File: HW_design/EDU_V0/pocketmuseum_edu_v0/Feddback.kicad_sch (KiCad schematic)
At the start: 18 parts

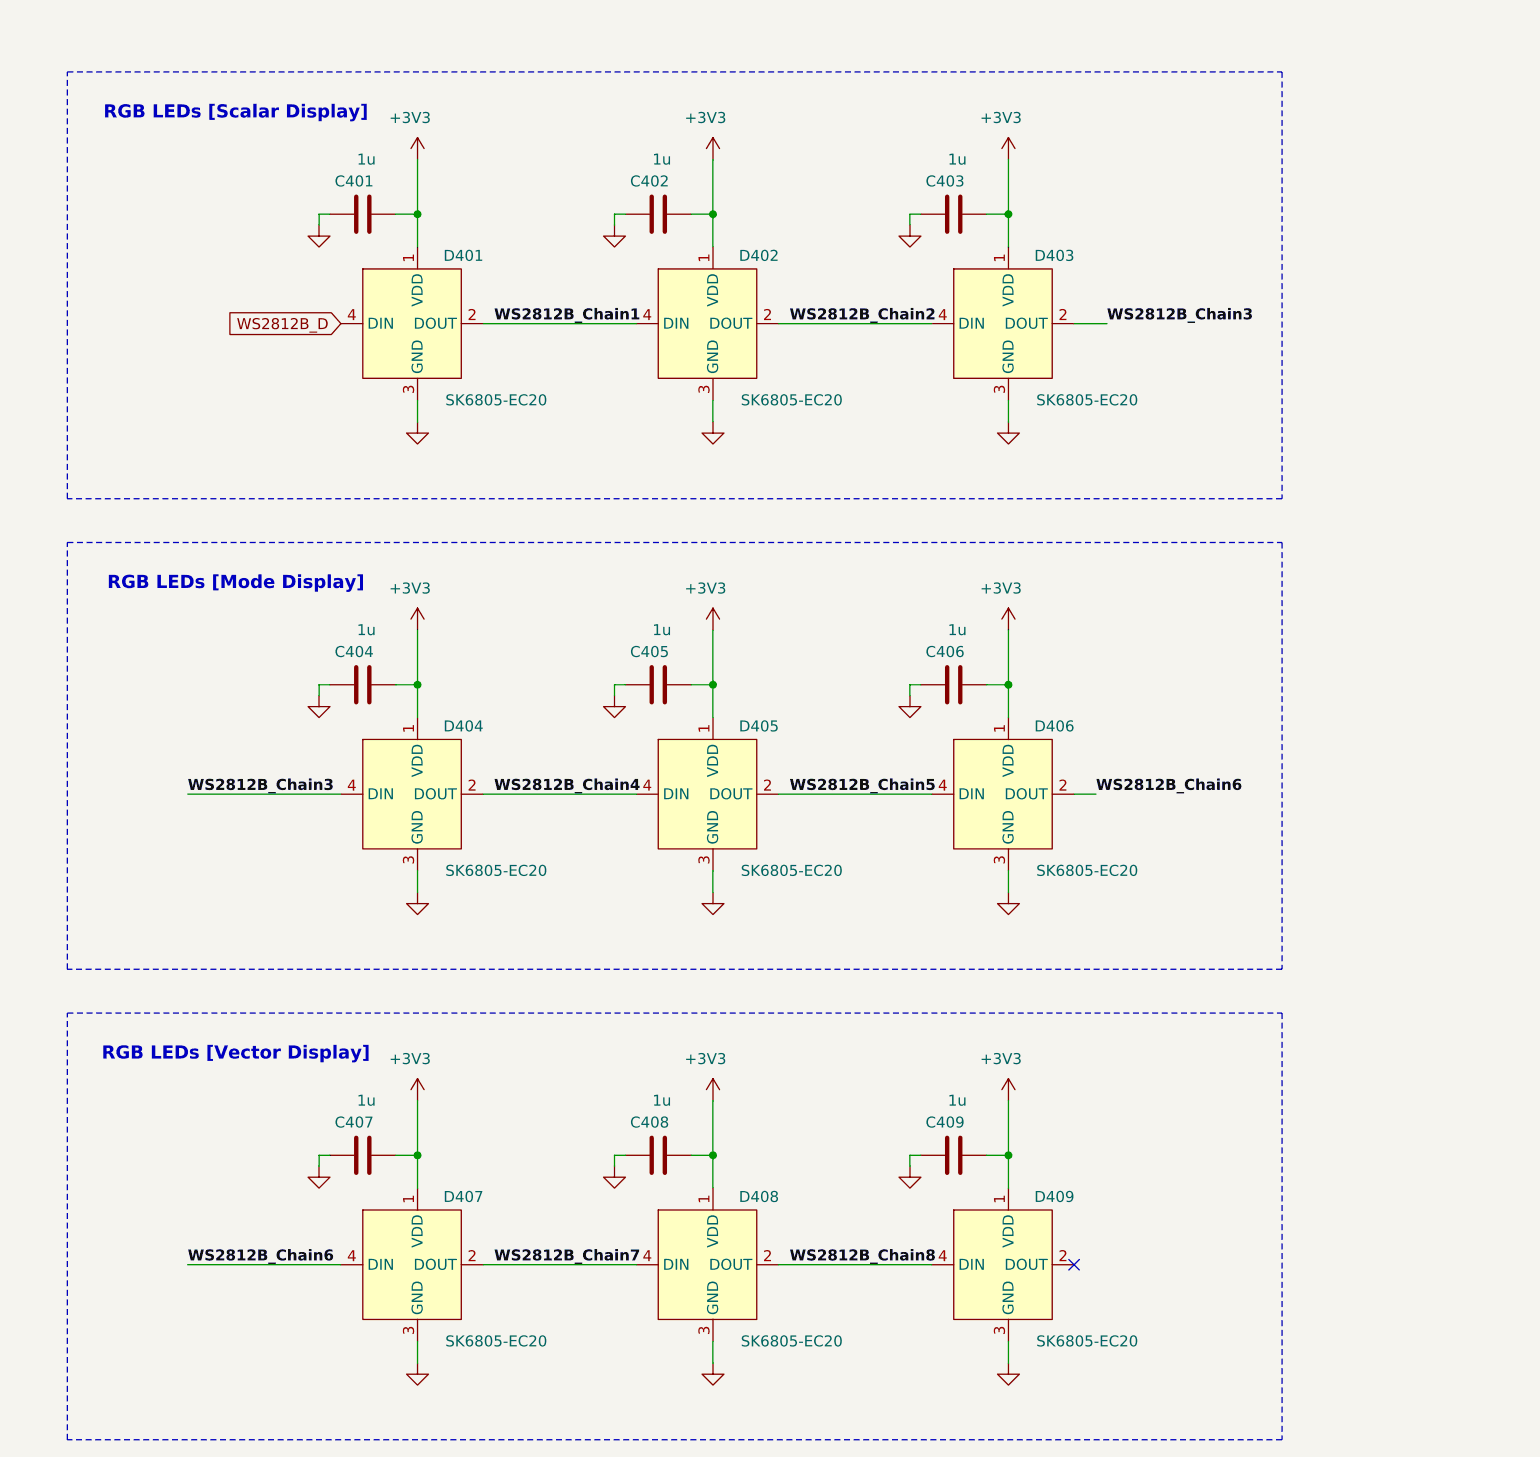
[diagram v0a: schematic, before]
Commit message: Diagram review complete
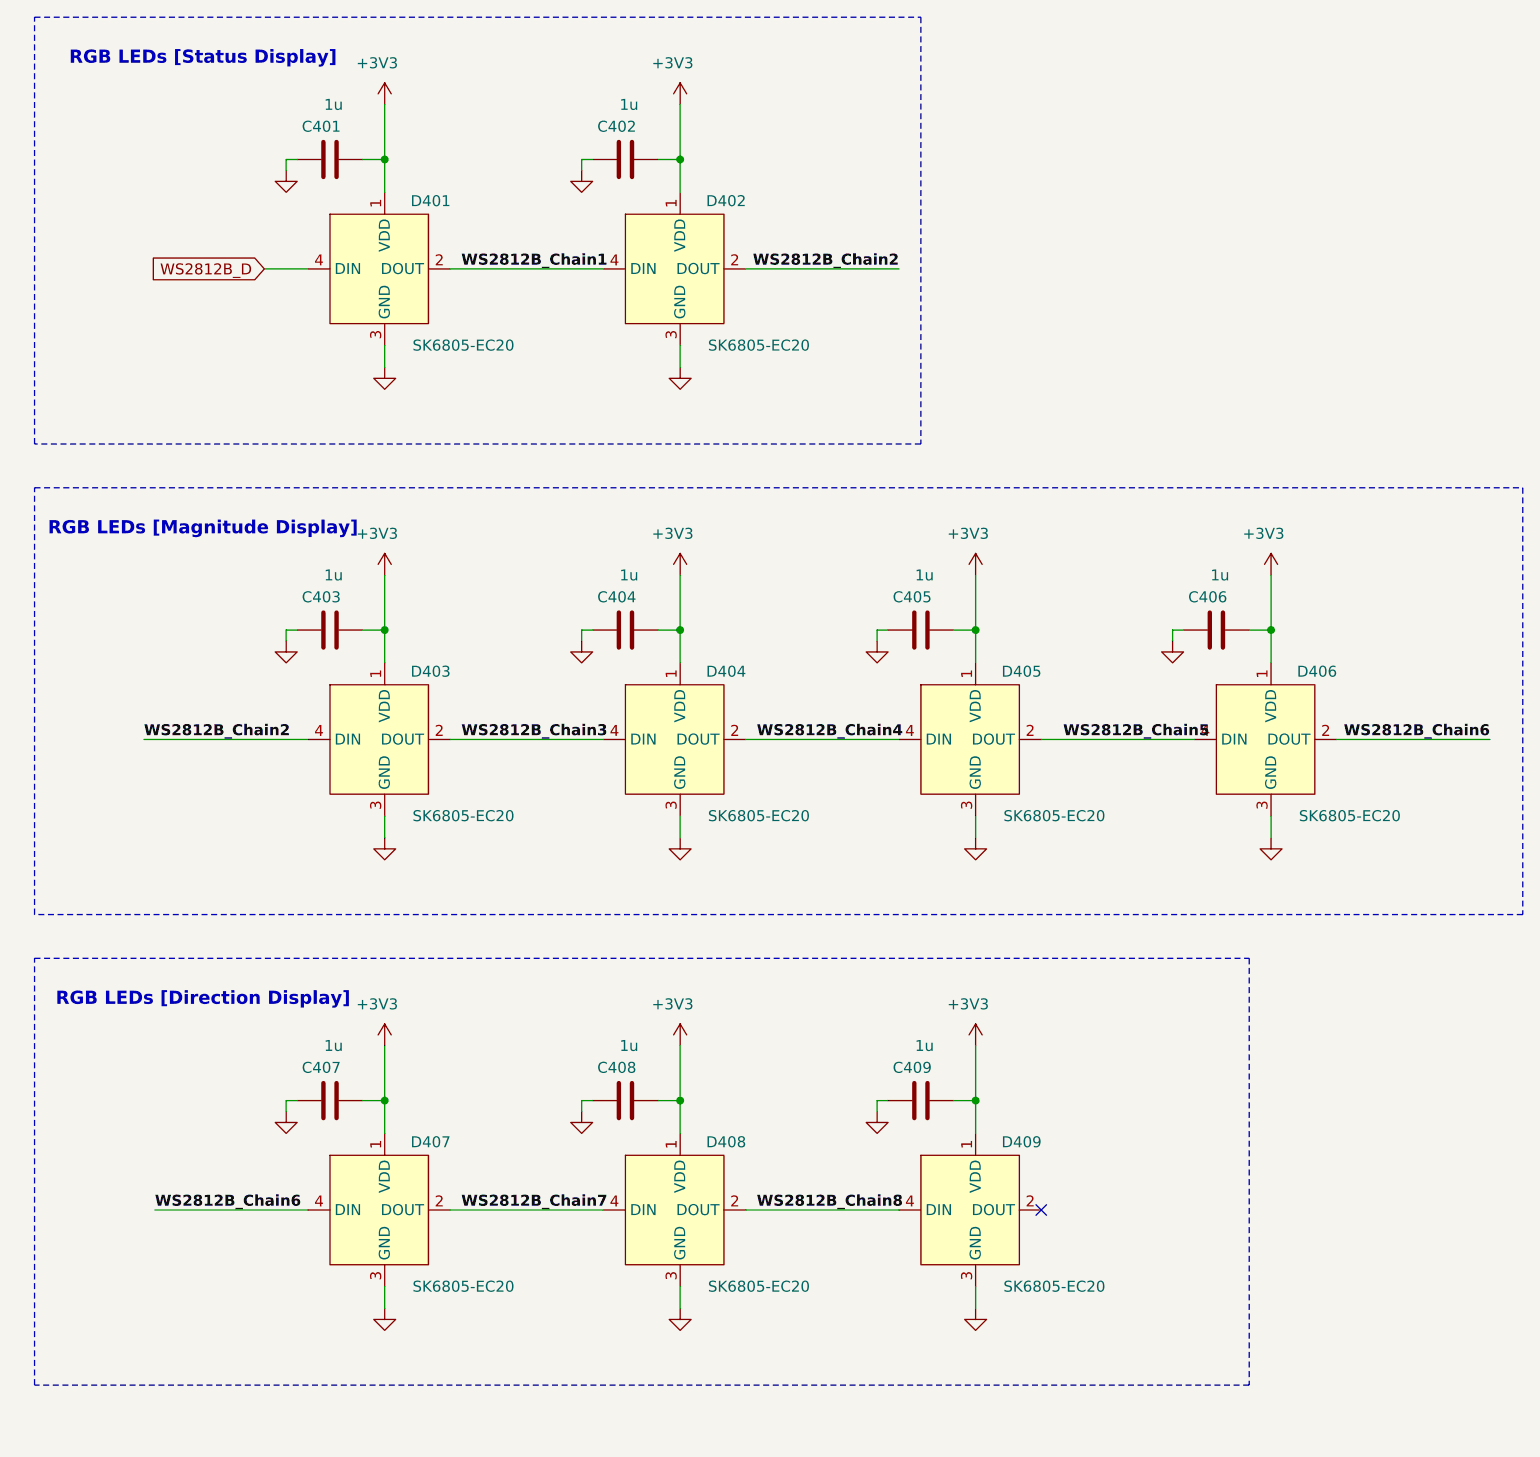
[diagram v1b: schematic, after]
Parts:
- renumbered C404 to C401, C405 to C402, C401 to C403, C402 to C404, C403 to C405, D404 to D401, D405 to D402, D401 to D403, D402 to D404, D403 to D405
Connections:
- net WS2812B_Chain1: now also D401.2 (DOUT), D402.4 (DIN); no longer D403.2 (DOUT), D404.4 (DIN)
- net WS2812B_Chain2: now also D402.2 (DOUT), D403.4 (DIN); no longer D404.2 (DOUT), D405.4 (DIN)
- net WS2812B_Chain3: now also D403.2 (DOUT), D404.4 (DIN); no longer D401.4 (DIN), D405.2 (DOUT)
- net WS2812B_Chain4: now also D404.2 (DOUT), D405.4 (DIN); no longer D401.2 (DOUT), D402.4 (DIN)
- net WS2812B_Chain5: now also D405.2 (DOUT); no longer D402.2 (DOUT)
- net WS2812B_D: now also D401.4 (DIN); no longer D403.4 (DIN)
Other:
- note added: "RGB LEDs [Direction Display]"
- note added: "RGB LEDs [Magnitude Display]"
- note added: "RGB LEDs [Status Display]"
- note removed: "RGB LEDs [Mode Display]"
- note removed: "RGB LEDs [Scalar Display]"
- note removed: "RGB LEDs [Vector Display]"
- moved on the sheet: C401, C402, C403, C404, C405, C407, C408, C409, D401, D402, D403, D404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
